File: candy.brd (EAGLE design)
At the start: 100 x 80 mm, 8 parts

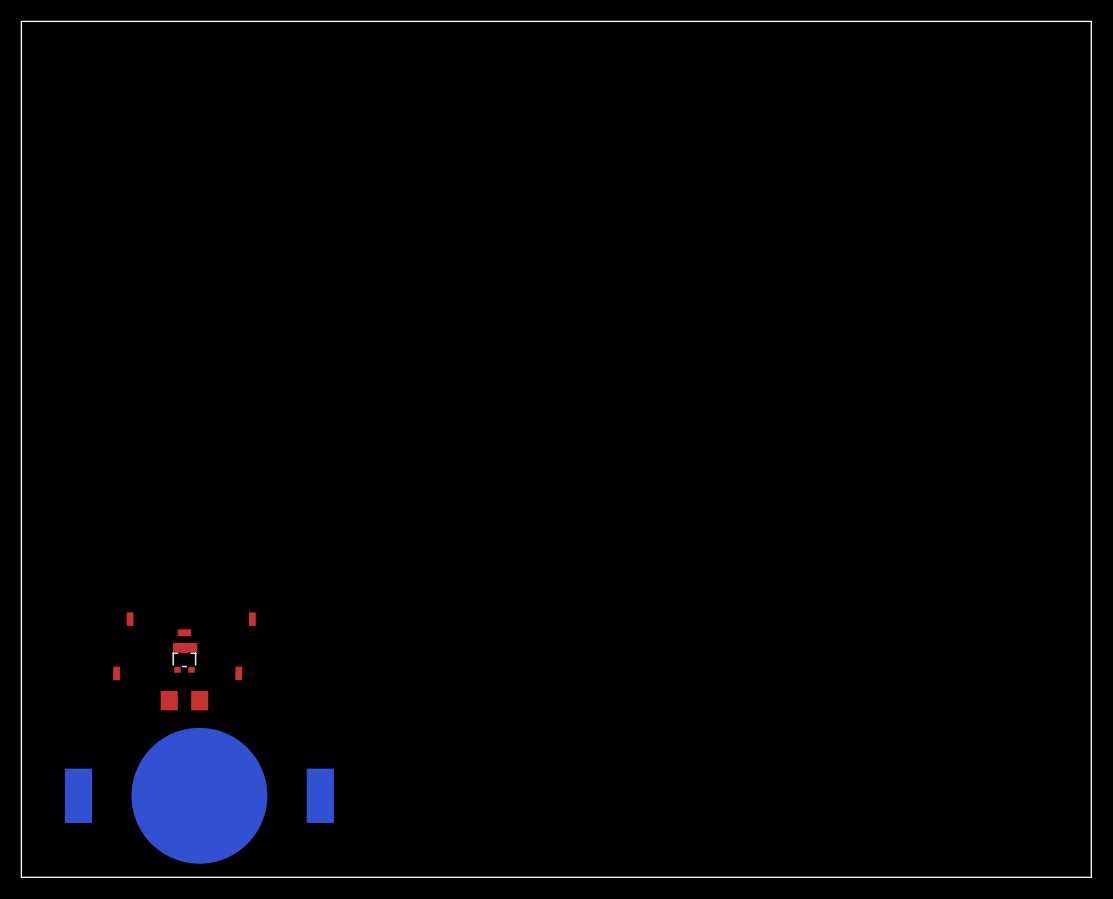
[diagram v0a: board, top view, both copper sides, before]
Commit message: sch
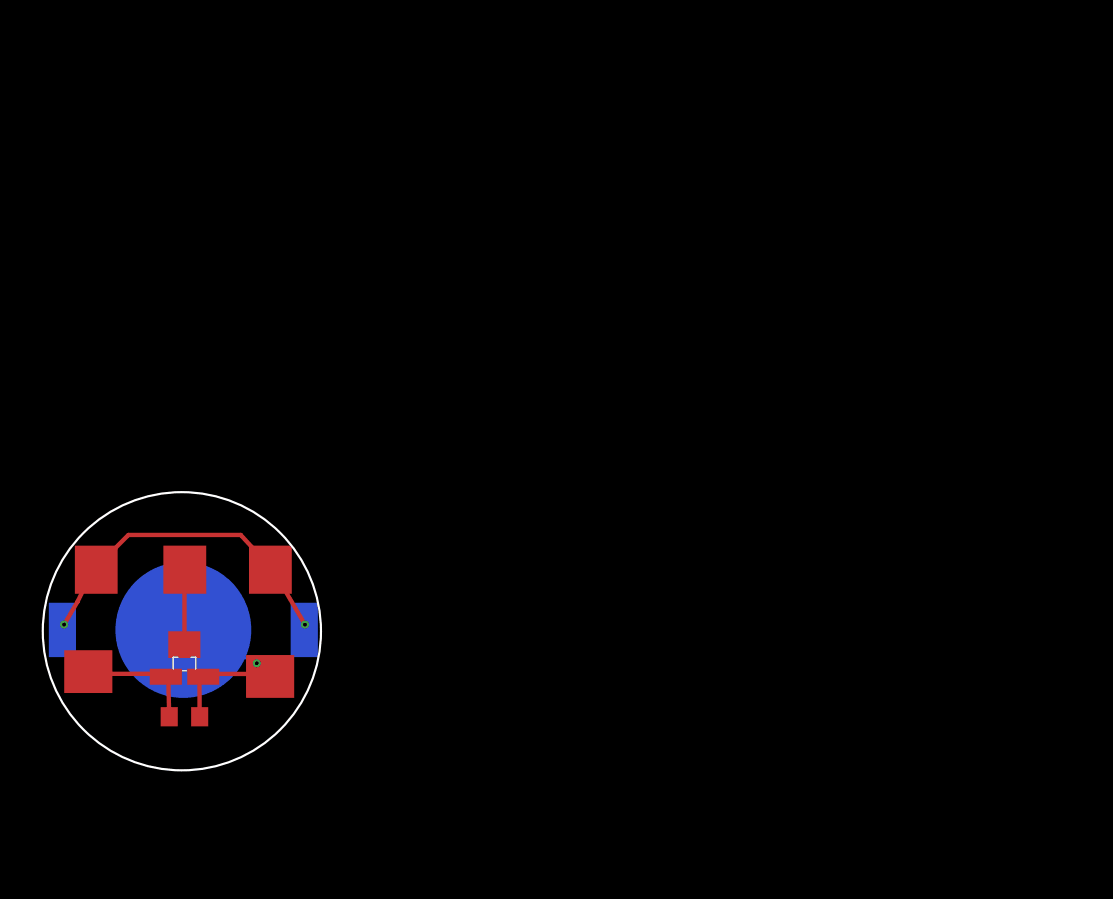
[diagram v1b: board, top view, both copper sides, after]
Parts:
- U$2: value N-MOSFET -> N-MOSFETREGULAR; device TinyTony_ShenzenReady:SOT323-CANDY -> TinyTony_ShenzenReady:SOT323
- moved U$7 15.6 mm to (15.1, 23.1)
- moved U$1 14.1 mm to (6.23, 19.0)
- moved U$4 11.7 mm to (15.2, 28.9)
- moved U$3 8.66 mm to (23.0, 19.0), turned to 0 degrees
- moved U$6 5.70 mm to (6.66, 28.6)
- moved U$5 4.92 mm to (23.6, 28.6)
- moved R1 1.50 mm to (15.2, 15.0), turned to 0 degrees
- moved U$2 0.38 mm to (15.2, 19.9)
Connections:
- net GND: now also U$2.2S; no longer U$2.3
- net N$1: now also U$2.1G; no longer U$2.2
- net N$3: now also U$2.3D; no longer U$2.1
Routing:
- net VCC: track 0.00 -> 32.3 mm, vias 0 -> 2
- net GND: track 0.00 -> 20.9 mm, vias 0 -> 1
- net N$1: track 0.00 -> 13.3 mm
- net N$3: track 0.00 -> 8.00 mm
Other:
- board size 100 x 80 mm -> 26 x 26 mm
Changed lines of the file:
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@@
 <setting verticaltext="up"/>
 </settings>
-<grid distance="50" unitdist="mil" unit="mil" style="lines" multiple="1" display="yes" altdistance="5" altunitdist="mil" altunit="mil"/>
+<grid distance="0.500000001" unitdist="mm" unit="mm" style="lines" multiple="1" display="yes" altdistance="5" altunitdist="mil" altunit="mil"/>
 <layers>
 <layer number="1" name="Top" color="4" fill="1" visible="yes" active="yes"/>
@@
 <layer number="27" name="tValues" color="7" fill="1" visible="yes" active="yes"/>
 <layer number="28" name="bValues" color="7" fill="1" visible="yes" active="yes"/>
-<layer number="29" name="tStop" color="7" fill="3" visible="no" active="yes"/>
-<layer number="30" name="bStop" color="7" fill="6" visible="no" active="yes"/>
-<layer number="31" name="tCream" color="7" fill="4" visible="no" active="yes"/>
+<layer number="29" name="tStop" color="7" fill="3" visible="yes" active="yes"/>
+<layer number="30" name="bStop" color="7" fill="6" visible="yes" active="yes"/>
+<layer number="31" name="tCream" color="7" fill="4" visible="yes" active="yes"/>
 <layer number="32" name="bCream" color="7" fill="5" visible="no" active="yes"/>
 <layer number="33" name="tFinish" color="6" fill="3" visible="no" active="yes"/>
@@
 <layer number="44" name="Drills" color="7" fill="1" visible="no" active="yes"/>
 <layer number="45" name="Holes" color="7" fill="1" visible="no" active="yes"/>
-<layer number="46" name="Milling" color="3" fill="1" visible="no" active="yes"/>
-<layer number="47" name="Measures" color="7" fill="1" visible="no" active="yes"/>
+<layer number="46" name="Milling" color="3" fill="1" visible="yes" active="yes"/>
+<layer number="47" name="Measures" color="7" fill="1" visible="yes" active="yes"/>
 <layer number="48" name="Document" color="7" fill="1" visible="yes" active="yes"/>
 <layer number="49" name="Reference" color="7" fill="1" visible="yes" active="yes"/>
@@
 <board>
 <plain>
-<wire x1="0" y1="0" x2="100" y2="0" width="0" layer="20"/>
-<wire x1="100" y1="0" x2="100" y2="80" width="0" layer="20"/>
-<wire x1="100" y1="80" x2="0" y2="80" width="0" layer="20"/>
-<wire x1="0" y1="80" x2="0" y2="0" width="0" layer="20"/>
+<rectangle x1="13.7287" y1="20.4978" x2="16.7287" y2="22.9978" layer="1"/>
+<rectangle x1="4.75" y1="26.75" x2="9.25" y2="30.75" layer="1" rot="R90"/>
+<rectangle x1="13.024040625" y1="26.752359375" x2="17.524040625" y2="30.752359375" layer="1" rot="R90"/>
+<rectangle x1="21.024040625" y1="26.752359375" x2="25.524040625" y2="30.752359375" layer="1" rot="R90"/>
+<rectangle x1="20.997640625" y1="16.774040625" x2="25.497640625" y2="20.774040625" layer="1" rot="R180"/>
+<rectangle x1="4.002359375" y1="17.225959375" x2="8.502359375" y2="21.225959375" layer="1"/>
+<circle x="15" y="23" radius="13" width="0.2032" layer="20"/>
+<rectangle x1="12" y1="18" x2="15" y2="19.5" layer="1"/>
+<rectangle x1="15.5" y1="18" x2="18.5" y2="19.5" layer="1"/>
+<rectangle x1="5" y1="26.5" x2="9" y2="31" layer="29"/>
+<rectangle x1="13.081" y1="26.416" x2="17.399" y2="31.115" layer="29"/>
+<rectangle x1="21.082" y1="26.416" x2="25.4" y2="31.242" layer="29"/>
+<rectangle x1="3.937" y1="17.145" x2="8.636" y2="21.336" layer="29"/>
+<rectangle x1="20.955" y1="16.637" x2="25.654" y2="20.828" layer="29"/>
+<rectangle x1="13.716" y1="20.447" x2="16.764" y2="23.114" layer="29"/>
+<rectangle x1="11.938" y1="17.907" x2="15.113" y2="19.558" layer="29"/>
+<rectangle x1="15.494" y1="17.907" x2="18.542" y2="19.558" layer="29"/>
+<rectangle x1="5" y1="26.5" x2="9" y2="31" layer="31"/>
+<rectangle x1="13.081" y1="26.416" x2="17.399" y2="31.115" layer="31"/>
+<rectangle x1="21.082" y1="26.416" x2="25.4" y2="31.242" layer="31"/>
+<rectangle x1="20.955" y1="16.637" x2="25.654" y2="20.828" layer="31"/>
+<rectangle x1="3.937" y1="17.145" x2="8.636" y2="21.336" layer="31"/>
+<rectangle x1="11.938" y1="17.907" x2="15.113" y2="19.558" layer="31"/>
+<rectangle x1="15.494" y1="17.907" x2="18.542" y2="19.558" layer="31"/>
+<rectangle x1="13.716" y1="20.447" x2="16.764" y2="23.114" layer="31"/>
 </plain>
 <attributes>
@@
 </autorouter>
 <elements>
-<element name="U$1" library="TinyTony_ShenzenReady" package="PADSMD" value="SMDPAD" x="20.32" y="19.05"/>
-<element name="U$2" library="TinyTony_ShenzenReady" package="SOT323-CANDY" value="N-MOSFET" x="15.24" y="20.32" smashed="yes"/>
-<element name="U$3" library="TinyTony_ShenzenReady" package="PADSMD" value="SMDPAD" x="15.24" y="22.86" rot="R90"/>
-<element name="U$4" library="TinyTony_ShenzenReady" package="PADSMD" value="SMDPAD" x="8.89" y="19.05"/>
-<element name="R1" library="adafruit" library_urn="urn:adsk.eagle:library:420" package="R1206" value="" x="15.24" y="16.51" smashed="yes" rot="R180">
-<attribute name="VALUE" x="16.637" y="18.923" size="1.27" layer="27" rot="R180"/>
+<element name="U$1" library="TinyTony_ShenzenReady" package="PADSMD" value="SMDPAD" x="6.2279375" y="19.019521875"/>
+<element name="U$2" library="TinyTony_ShenzenReady" package="SOT323" value="N-MOSFETREGULAR" x="15.24" y="19.939" smashed="yes"/>
+<element name="U$3" library="TinyTony_ShenzenReady" package="PADSMD" value="SMDPAD" x="23.000978125" y="19.006821875"/>
+<element name="U$4" library="TinyTony_ShenzenReady" package="PADSMD" value="SMDPAD" x="15.24" y="28.86"/>
+<element name="R1" library="adafruit" library_urn="urn:adsk.eagle:library:420" package="R1206" value="" x="15.24" y="15.01" smashed="yes">
+<attribute name="VALUE" x="13.843" y="12.597" size="1.27" layer="27"/>
 </element>
-<element name="U$5" library="TinyTony_ShenzenReady" package="PADSMD" value="SMDPAD" x="21.59" y="24.13"/>
-<element name="U$6" library="TinyTony_ShenzenReady" package="PADSMD" value="SMDPAD" x="10.16" y="24.13"/>
-<element name="U$7" library="TinyTony_ShenzenReady" package="LINX" value="" x="16.637" y="7.62" rot="MR0"/>
+<element name="U$5" library="TinyTony_ShenzenReady" package="PADSMD" value="SMDPAD" x="23.59" y="28.63"/>
+<element name="U$6" library="TinyTony_ShenzenReady" package="PADSMD" value="SMDPAD" x="6.66" y="28.63"/>
+<element name="U$7" library="TinyTony_ShenzenReady" package="LINX" value="" x="15.137" y="23.12" rot="MR0"/>
 </elements>
 <signals>
 <signal name="N$1">
-<contactref element="U$2" pad="2"/>
+<contactref element="U$2" pad="1G"/>
 <contactref element="U$1" pad="P$1"/>
 <contactref element="R1" pad="1"/>
-<wire x1="15.89" y1="19.395" x2="16.662" y2="16.51" width="0" layer="19" extent="1-1"/>
-<wire x1="20.32" y1="19.05" x2="15.89" y2="19.395" width="0" layer="19" extent="1-1"/>
+<wire x1="6.2279375" y1="19.019521875" x2="14.584478125" y2="19.019521875" width="0.4064" layer="1"/>
+<wire x1="14.584478125" y1="19.019521875" x2="14.59" y2="19.014" width="0.2032" layer="1"/>
+<wire x1="14.59" y1="19.014" x2="13.716" y2="19.05" width="0.4064" layer="1"/>
+<wire x1="13.716" y1="19.05" x2="13.818" y2="15.01" width="0.4064" layer="1"/>
 </signal>
 <signal name="N$3">
-<contactref element="U$2" pad="1"/>
+<contactref element="U$2" pad="3D"/>
 <contactref element="U$4" pad="P$1"/>
-<wire x1="8.89" y1="19.05" x2="14.59" y2="19.395" width="0" layer="19" extent="1-1"/>
+<wire x1="15.24" y1="20.864" x2="15.24" y2="28.86" width="0.4064" layer="1"/>
 </signal>
 <signal name="GND">
 <contactref element="U$7" pad="P$1-"/>
-<contactref element="U$2" pad="3"/>
+<contactref element="U$2" pad="2S"/>
 <contactref element="U$3" pad="P$1"/>
 <contactref element="R1" pad="2"/>
-<wire x1="13.818" y1="16.51" x2="16.637" y2="7.62" width="0" layer="19" extent="1-1"/>
-<wire x1="15.24" y1="21.245" x2="13.818" y2="16.51" width="0" layer="19" extent="1-1"/>
-<wire x1="15.24" y1="22.86" x2="15.24" y2="21.245" width="0" layer="19" extent="1-1"/>
+<wire x1="22.000009375" y1="19.00783125" x2="23.000978125" y2="19.006821875" width="0.4064" layer="1"/>
+<wire x1="15.89" y1="19.014" x2="16.637" y2="19.05" width="0.4064" layer="1"/>
+<wire x1="16.637" y1="19.05" x2="16.662" y2="15.01" width="0.4064" layer="1"/>
+<wire x1="15.89" y1="19.014" x2="22.000009375" y2="19.00783125" width="0.4064" layer="1"/>
+<wire x1="23.000978125" y1="19.006821875" x2="21.971" y2="19.939" width="0.4064" layer="1"/>
+<wire x1="21.971" y1="19.939" x2="22" y2="20" width="0.2032" layer="1"/>
+<via x="22" y="20" extent="1-16" drill="0.35"/>
+<wire x1="22" y1="20" x2="15.137" y2="23.12" width="0.2032" layer="16"/>
 </signal>
 <signal name="VCC">
@@
 <contactref element="U$7" pad="P$3+"/>
 <contactref element="U$7" pad="P$2+"/>
-<wire x1="27.94" y1="7.62" x2="5.334" y2="7.62" width="0" layer="19" extent="1-1"/>
-<wire x1="21.59" y1="24.13" x2="27.94" y2="7.62" width="0" layer="19" extent="1-1"/>
-<wire x1="10.16" y1="24.13" x2="21.59" y2="24.13" width="0" layer="19" extent="1-1"/>
+<wire x1="23.59" y1="28.63" x2="26.5" y2="23.627" width="0.4064" layer="1"/>
+<via x="26.5" y="23.627" extent="1-16" drill="0.35"/>
+<wire x1="26.5" y1="23.627" x2="26.44" y2="23.12" width="0.4064" layer="16"/>
+<wire x1="3.834" y1="23.12" x2="3.992" y2="23.627" width="0.4064" layer="16"/>
+<via x="3.992" y="23.627" extent="1-16" drill="0.35"/>
+<wire x1="5.238" y1="25.746" x2="3.992" y2="23.627" width="0.4064" layer="1"/>
+<wire x1="6.66" y1="28.63" x2="5.238" y2="25.746" width="0.4064" layer="1"/>
+<wire x1="6.66" y1="28.63" x2="10" y2="32" width="0.4064" layer="1"/>
+<wire x1="10" y1="32" x2="20.5" y2="32" width="0.4064" layer="1"/>
+<wire x1="20.5" y1="32" x2="23.59" y2="28.63" width="0.4064" layer="1"/>
 </signal>
 </signals>
@@
 with this version.
 </note>
+<note version="8.3" severity="warning">
+Since Version 8.3, EAGLE supports URNs for individual library
+assets (packages, symbols, and devices). The URNs of those assets
+will not be understood (or retained) with this version.
+</note>
 </compatibility>
